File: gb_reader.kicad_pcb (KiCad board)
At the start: 2 copper layers, 46 parts, among them J1 USB_B_Micro, J2 Conn_01x09, J3 Conn_01x04, J4 Conn_01x32, J5 Conn_01x32_MountingPin, SW1 SW_Push, SW2 SW_Push, SW3 SW_Push, SW4 SW_Push, U1 STM32F103RFTx, U2 TLV70233_SOT23-5, U3 TXB0108PWR, U4 TXB0108PWR, U5 TXB0108PWR, U6 TXB0108PWR, Y1 32kHz

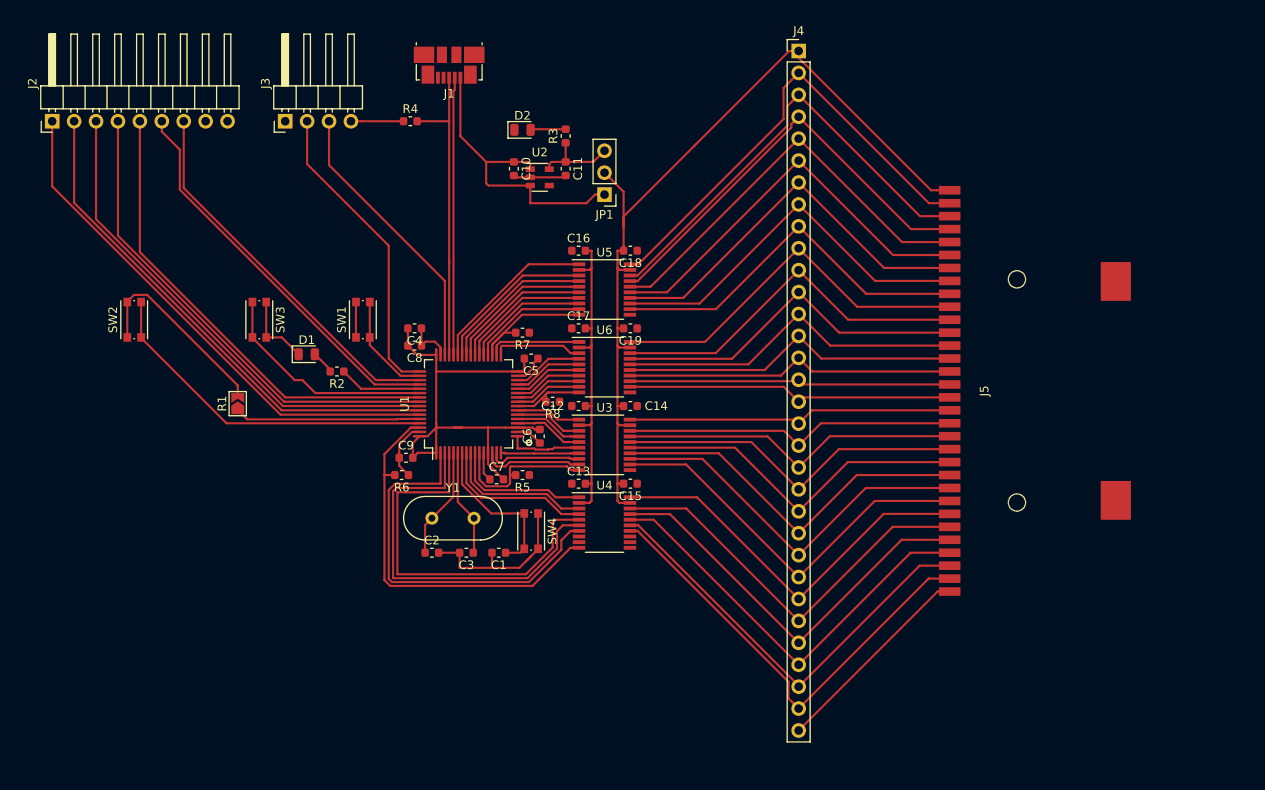
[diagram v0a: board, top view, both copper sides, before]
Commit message: blo
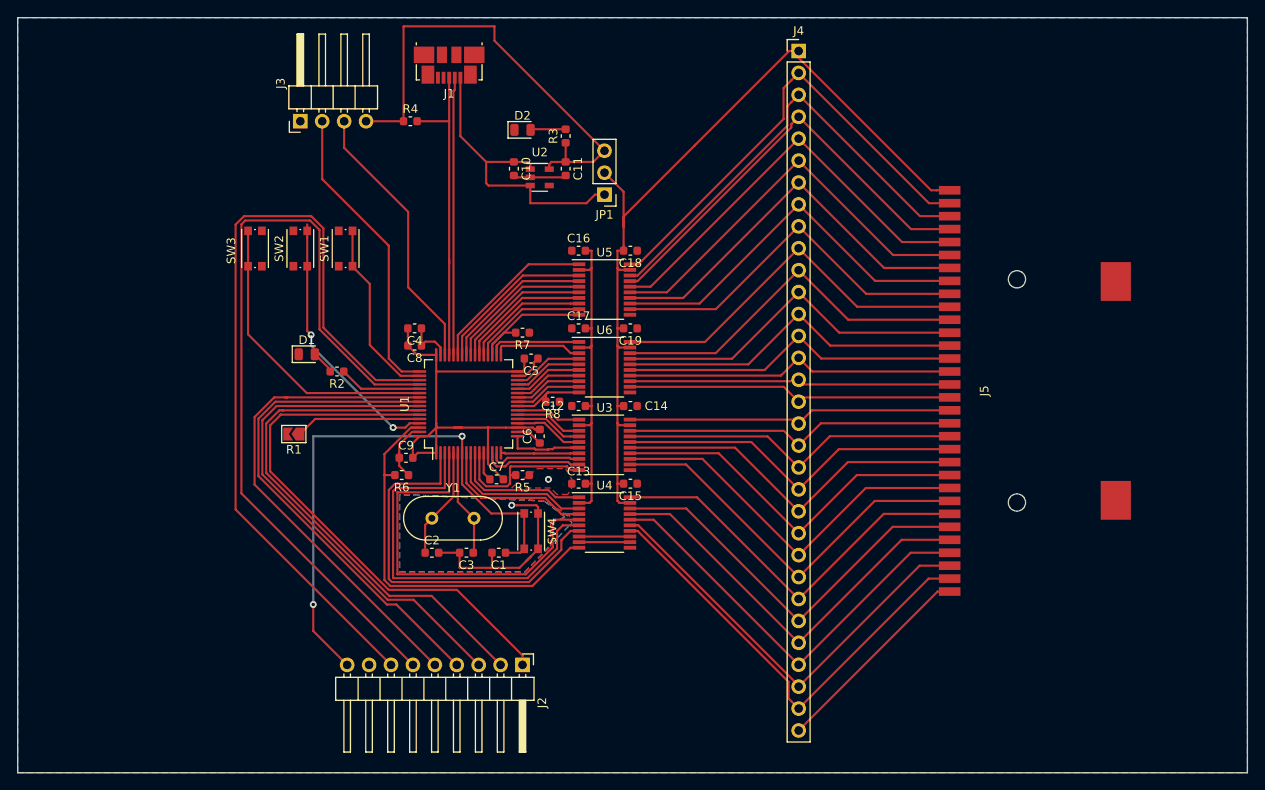
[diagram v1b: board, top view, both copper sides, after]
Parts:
- moved J2 83.3 mm to (143.5, 117.5), turned to 270 degrees
- moved SW2 20.9 mm to (117.8, 69.2)
- moved SW1 8.49 mm to (123.0, 69.2)
- moved SW3 8.27 mm to (112.5, 69.2)
- moved R1 7.39 mm to (117.0, 90.8), turned to 180 degrees
- moved J3 1.75 mm to (117.8, 54.5)
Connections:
- U4 pad 12: (no net) -> GND
- U4 pad 13: (no net) -> GND
- U4 pad 8: (no net) -> GND
- U4 pad 9: (no net) -> GND
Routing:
- net UART4_TX: track 44.3 -> 94.8 mm
- net UART4_RX: track 45.9 -> 94.7 mm
- net /NRST: track 18.7 -> 66.0 mm, vias 0 -> 2
- net +3V3: track 111.0 -> 150.5 mm
- net GND: track 109.4 -> 89.3 mm, vias 0 -> 2
- net /T-B: track 40.5 -> 31.0 mm, vias 0 -> 2
- net /T-A: track 12.2 -> 21.3 mm
- net /T-C: track 26.2 -> 34.7 mm
- net /BOOT0: track 21.6 -> 14.6 mm
- net SPI_SCK: track 54.6 -> 57.7 mm
- net SPI_MISO: track 56.2 -> 58.2 mm
- net SPI_MOSI: track 57.8 -> 59.4 mm
- net I2C_SDA: track 61.1 -> 62.4 mm
- net I2C_SCL: track 59.4 -> 60.7 mm
- net SWCLK: track 35.6 -> 34.9 mm
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- added copper zone on B.Cu, net GND
- added copper zone on F.Cu, net GND
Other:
- board outline added: 142.5 x 87.5 mm
